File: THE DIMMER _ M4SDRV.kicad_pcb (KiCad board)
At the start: 4 copper layers, 37 x 23.8 mm, 89 parts, among them J1 Conn_01x01, J10 GS2, J2 USB_B_Micro, J3 Conn_01x05, J4 Conn_01x02, J5 Conn_01x01, J6 Conn_01x01, J7 Conn_01x04, J8 Conn_01x02, J9 Conn_01x04, U1 ATSAMD51J19A-M, U10 DRV50153A, U11 DRV50152A, U12 MAX40056_uMAX8, U13 MAX40056_uMAX8, U14 TMC2209-LA, U15 MIC4605-2YMT, U16 MIC4605-2YMT, U2 MIC4605-2YMT, U3 LM2672M-12, U4 BSC0925NDATMA1, U5 BSC0925NDATMA1, U6 BSC0925NDATMA1, U7 MAX40056_uMAX8, U8 NCP170, U9 DRV50152A, Y1 Crystal_GND2_Small

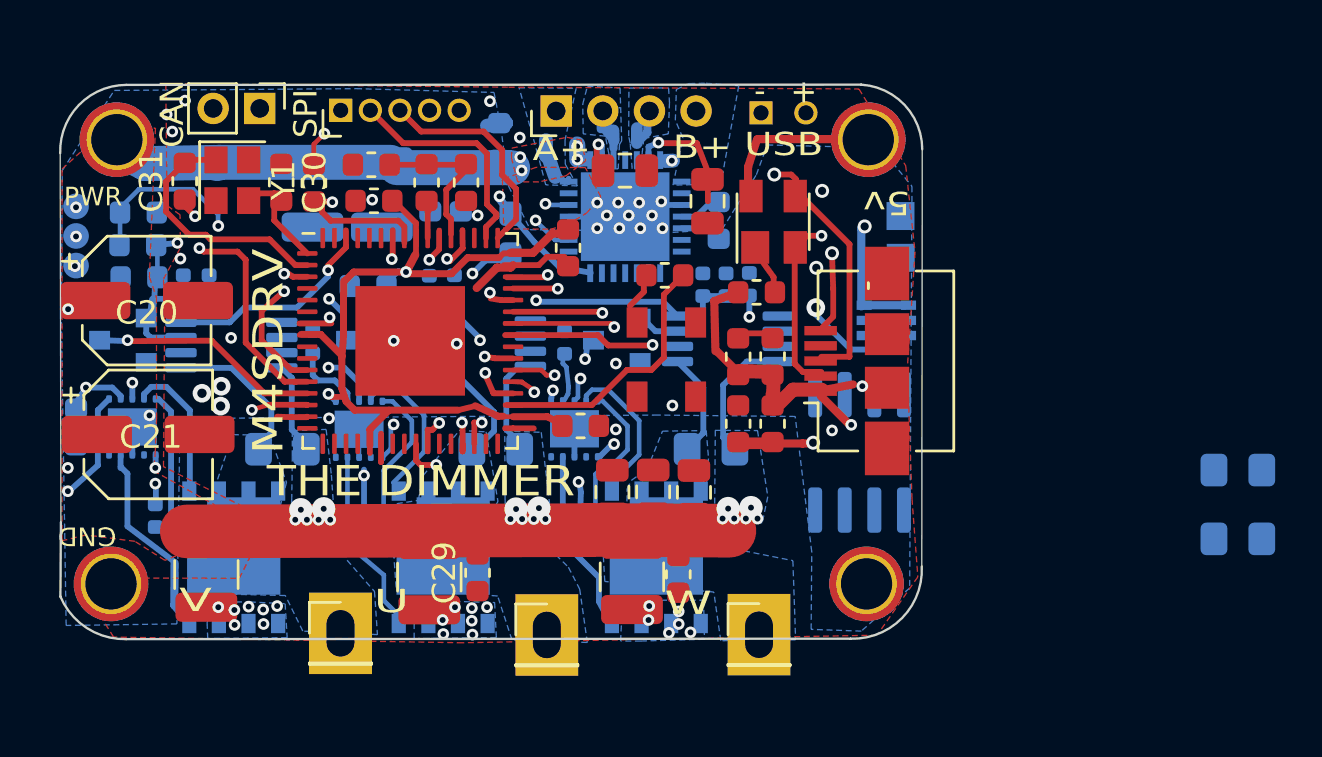
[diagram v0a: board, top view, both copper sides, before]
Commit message: update
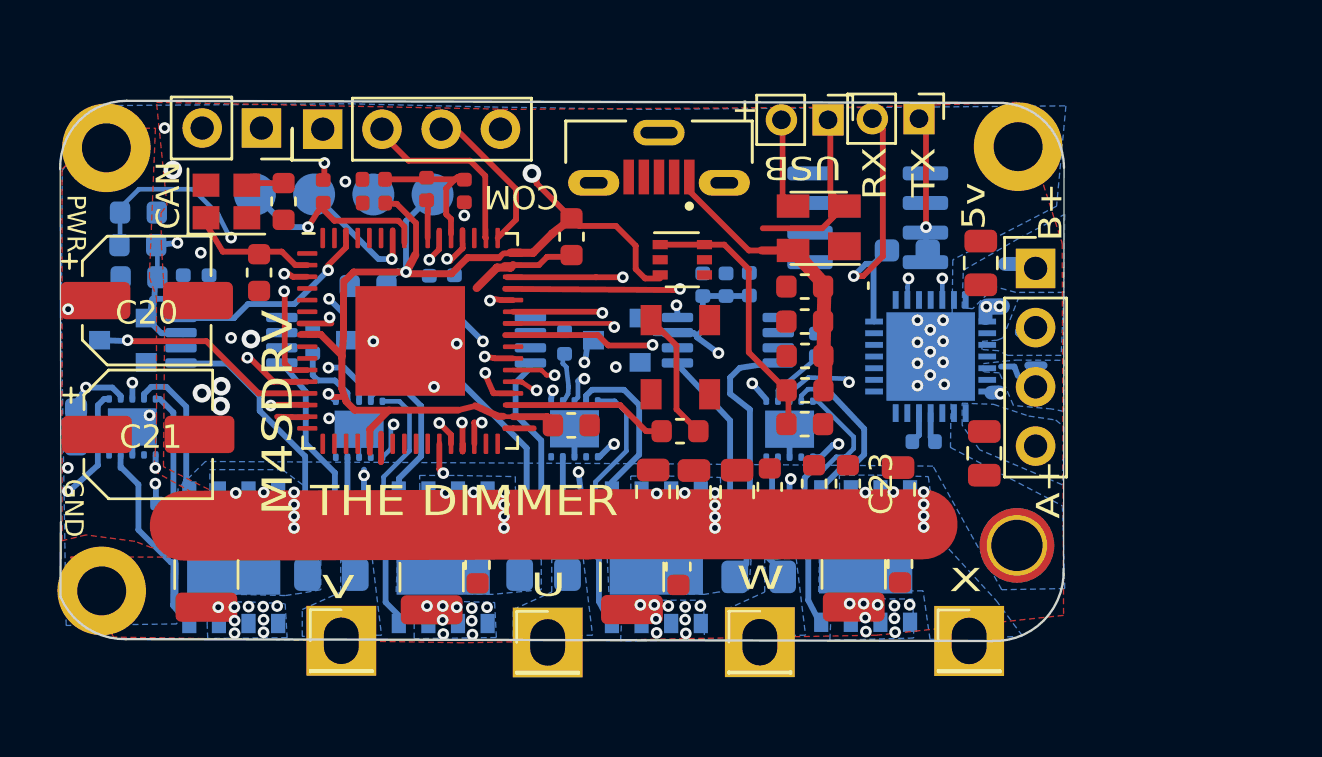
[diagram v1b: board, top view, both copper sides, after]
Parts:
- removed C10, C9: 10uF, Capacitor_SMD:C_1210_3225Metric
- removed C24: 10nF, Capacitor_SMD:C_0603_1608Metric
- removed J10: GS2, LED_SMD:Solder joint
- removed R12, R16: 0.02ohm, Resistor_SMD:R_0805_2012Metric_Pad1.15x1.40mm_HandSolder
- added C22: 1uF7, Capacitor_SMD:C_0603_1608Metric, F.Cu at (94.0, 75.0)
- added C25: 4.7uF, Capacitor_SMD:C_0805_2012Metric, F.Cu at (99.5, 75.1)
- added C28: 1uF, Capacitor_SMD:C_0603_1608Metric, F.Cu at (99.5, 78.3)
- added C44: 1uF, Capacitor_SMD:C_0402_1005Metric, B.Cu at (96.0, 68.9)
- added C45: 1uF, Capacitor_SMD:C_0402_1005Metric, B.Cu at (94.8, 76.5)
- added C8: 10uF, Capacitor_SMD:C_1210_3225Metric, F.Cu at (97.6, 78.7)
- added J11: Conn_01x01, Connector_PinHeader_2.54mm:PinHeader_1x01_P2.54mm_Vertical, F.Cu at (102.5, 81.6)
- added J12: Conn_01x02, Connector_PinHeader_2.00mm:PinHeader_1x02_P2.00mm_Vertical, F.Cu at (100.4, 59.2)
- added U17: MIC4605-2YMT, LED_SMD:MIC4605, B.Cu at (94.8, 72.5)
- added U18: BSC0925NDATMA1, Package_SON:Infineon_PG-TISON-8-2, B.Cu at (99.7, 80.3)
- C11, C16, C19, C2: footprint Capacitor_SMD:C_0603_1608Metric -> Capacitor_SMD:C_0402_1005Metric
- C22, C23, U8: moved to F.Cu
- J2: footprint Connector_USB:USB_Micro-B_Amphenol_10104110_Horizontal -> molex_usb_vert:MOLEX_1051330001
- J3: footprint Connector_PinHeader_1.27mm:PinHeader_1x05_P1.27mm_Vertical -> Connector_PinHeader_2.54mm:PinHeader_1x04_P2.54mm_Vertical
- J4: footprint Connector_PinHeader_2.00mm:PinHeader_1x02_P2.00mm_Vertical -> Connector_PinSocket_2.54mm:PinSocket_1x02_P2.54mm_Vertical
- J7: footprint Connector_PinHeader_2.00mm:PinHeader_1x04_P2.00mm_Vertical -> Connector_PinHeader_2.54mm:PinHeader_1x04_P2.54mm_Vertical
- J8: footprint Connector_PinHeader_1.27mm:PinHeader_1x02_P1.27mm_Vertical -> Connector_PinHeader_2.00mm:PinHeader_1x02_P2.00mm_Vertical
- L1: footprint Inductor_SMD:L_0603_1608Metric -> Inductor_SMD:L_0402_1005Metric
- R6: footprint Resistor_SMD:R_0603_1608Metric -> Resistor_SMD:R_0402_1005Metric
- moved R2 38.9 mm to (75.2, 78.7)
- moved R3 30.1 mm to (84.3, 78.7)
- moved C23 21.8 mm to (97.3, 74.8), turned to -90 degrees
- moved J7 21.6 mm to (105.4, 65.6), turned to 0 degrees
- moved C22 19.9 mm to (95.9, 74.8)
- moved R21 17.0 mm to (99.9, 64.8), turned to 0 degrees
- moved R19 16.1 mm to (103.2, 73.5)
- moved R20 15.8 mm to (103.0, 65.4), turned to -90 degrees
- moved U14 14.4 mm to (100.9, 69.4), turned to 90 degrees
- moved J9 13.1 mm to (77.0, 62.4), turned to 0 degrees
- moved C19 12.9 mm to (100.6, 73.0), turned to 180 degrees
- moved R8 12.5 mm to (93.5, 78.8)
- moved J2 11.4 mm to (89.2, 61.9), turned to 180 degrees
- moved U3 10.1 mm to (98.2, 63.4), turned to 180 degrees
- moved U8 9.13 mm to (90.2, 65.2), turned to 0 degrees
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- renumbered U7 to U12, U12 to U7
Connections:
- net TCC0_CH2/Switch 3 renamed TCC0_CH2/CAN0Switch 3
- R2 pad 1: +12V -> V
- R2 pad 2: +12V -> V
- R3 pad 1: +12V -> U
- R3 pad 2: +12V -> U
- R8 pad 1: +12V -> W
- R8 pad 2: +12V -> W
- U1 pad 25: CAN1_TX -> Net-(U1-Pad25)
- U1 pad 26: CAN1_RX -> CAN1_STANDBY
- U1 pad 27: Net-(U1-Pad27) -> CAN1_TX
- U1 pad 28: Net-(U1-Pad28) -> CAN1_RX
- U12 pad 1: +12V -> V
- U12 pad 8: +12V -> V
- U13 pad 1: +12V -> U
- U13 pad 8: +12V -> U
- U15 pad 11: GND -> (no net)
- U16 pad 11: GND -> (no net)
- U2 pad 11: GND -> (no net)
- U7 pad 1: +12V -> W
- U7 pad 8: +12V -> W
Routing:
- net +12V: track 80.0 -> 44.6 mm, vias 24 -> 29
- net UART_TX: track 11.8 -> 35.4 mm
- net V: track 9.62 -> 31.6 mm
- net W: track 10.8 -> 32.2 mm
- net U: track 11.9 -> 33.3 mm
- net VBUS: track 30.8 -> 12.8 mm, vias 2 -> 0
- net UART_RX: track 17.4 -> 33.0 mm
- net GND: track 31.2 -> 16.8 mm, vias 56 -> 65
- net Net-(C45-Pad1): track 0.00 -> 12.3 mm, vias 0 -> 2
- net X: track 0.00 -> 11.5 mm
- net SWDIO: track 17.1 -> 5.67 mm, vias 2 -> 1
- net SWCLK: track 19.3 -> 8.90 mm, vias 2 -> 1
- net D+: track 28.7 -> 18.8 mm, vias 2 -> 1
- net A3: track 34.2 -> 25.2 mm
- net STEP: track 11.5 -> 20.5 mm
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- added copper zone on B.Cu, net X
- removed copper zone on In1.Cu, net +12V
- removed copper zone on In2.Cu, net +12V
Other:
- board size 37 x 23.8 mm -> 43.1 x 23.2 mm
- board text added: "CLK"
- board text added: "COM"
- board text added: "DIO"
- board text added: "RX"
- board text added: "TX"
- board text added: "X"
- board text removed: "-"
- board text removed: "SPI"

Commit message: Dev.
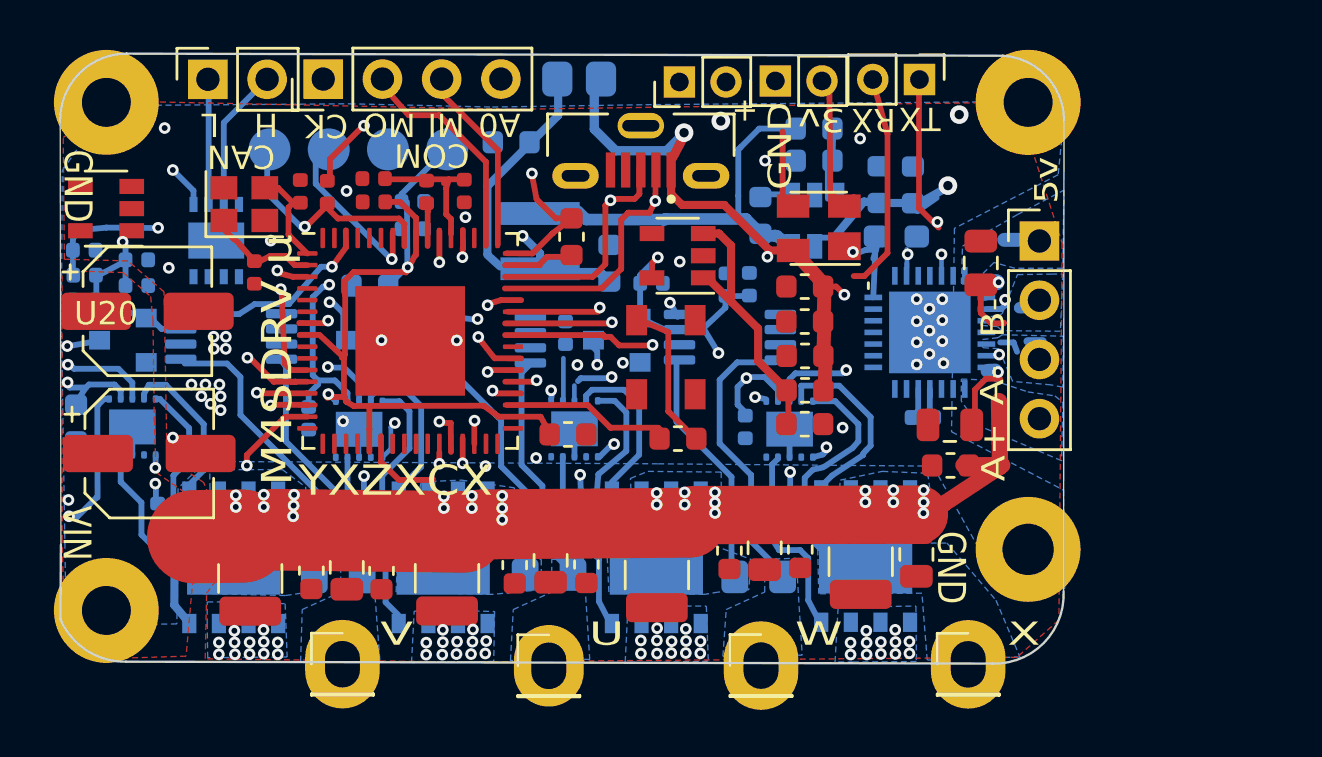
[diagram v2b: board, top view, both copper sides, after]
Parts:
- removed the C8 at (97.6, 78.7)
- added C10: 10uF, Capacitor_SMD:C_1210_3225Metric, F.Cu at (97.9, 78.2)
- added C24: 10nF, Capacitor_SMD:C_0603_1608Metric, F.Cu at (92.2, 77.7)
- added C46: 2.2uF, Capacitor_SMD:C_0603_1608Metric, B.Cu at (98.6, 62.0)
- added C47: 200nF, Capacitor_SMD:C_0603_1608Metric, B.Cu at (100.1, 62.0)
- added C49: 0.1uF, Capacitor_SMD:C_0603_1608Metric, B.Cu at (93.6, 63.3)
- added C50: 200nF, Capacitor_SMD:C_0603_1608Metric, B.Cu at (87.1, 65.4)
- added C51: 200nF, Capacitor_SMD:C_0603_1608Metric, B.Cu at (82.9, 60.2)
- added J10: GS2, Resistor_SMD:R_0805_2012Metric, B.Cu at (85.8, 57.5)
- added J8: Conn_01x02, Connector_PinHeader_2.00mm:PinHeader_1x02_P2.00mm_Vertical, F.Cu at (90.1, 57.6)
- added L2: 33uH, Inductor_SMD:L_Coilcraft_XxL4020, B.Cu at (84.1, 64.4)
- added R1: 100k, Resistor_SMD:R_0603_1608Metric, B.Cu at (95.9, 59.6)
- added R7: 11.11k, Resistor_SMD:R_0603_1608Metric, B.Cu at (95.9, 61.0)
- added U19: MCP2562FD-E_SN, Package_DFN_QFN:DFN-8-1EP_3x3mm_P0.65mm_EP1.55x2.4mm, B.Cu at (70.2, 64.4)
- added U20: LF15_TO220, Package_TO_SOT_SMD:SOT-23-5, F.Cu at (65.5, 63.0)
- C1, C13, C30, C31: footprint Capacitor_SMD:C_0603_1608Metric -> Capacitor_SMD:C_0402_1005Metric
- R5: footprint Resistor_SMD:R_0603_1608Metric -> Resistor_SMD:R_0402_1005Metric
- U10: value DRV50153A -> DRV5053
- U11, U9: value DRV50152A -> DRV5053
- U3: value LM2672M-12 -> LMR50410; footprint Package_SO:SOIC-8_3.9x4.9mm_P1.27mm -> Package_TO_SOT_SMD:SOT-23-6
- U8: value NCP170 -> MIC5219-3.6; footprint Package_TO_SOT_SMD:SOT-363_SC-70-6 -> Package_TO_SOT_SMD:SOT-23-5
- moved C25 23.9 mm to (75.8, 78.4), turned to 90 degrees
- moved H3 21.1 mm to (65.5, 58.4)
- moved C23 20.3 mm to (77.3, 78.6), turned to 90 degrees
- moved C22 20.0 mm to (74.3, 78.6), turned to 90 degrees
- moved H2 19.8 mm to (65.5, 80.3)
- moved C26 8.14 mm to (100.2, 77.9), turned to 90 degrees
- moved C28 7.02 mm to (83.0, 78.3)
- moved C25 6.81 mm to (84.6, 78.1), turned to 90 degrees
- moved C27 5.35 mm to (93.7, 77.6), turned to 90 degrees
- moved C28 4.75 mm to (101.7, 74.1), turned to 0 degrees
- moved C29 4.67 mm to (86.1, 78.3)
- moved C44 4.66 mm to (92.9, 72.4), turned to -90 degrees
- moved C43 4.06 mm to (78.6, 62.7), turned to 180 degrees
- moved C33 3.28 mm to (74.2, 72.0), turned to -90 degrees
- moved J4 3.10 mm to (69.9, 57.5), turned to 90 degrees
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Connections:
- C18 pad 2: +12V -> VIN
- C20 pad 1: +12V -> VIN
- C21 pad 1: +12V -> VIN
- C22 pad 2: +12V -> VIN (x2)
- C23 pad 2: +12V -> VIN
- C25 pad 2: +12V -> VIN (x2)
- C26 pad 2: +12V -> VIN
- C27 pad 2: +12V -> VIN
- C28 pad 2: +12V -> VIN (x2)
- C29 pad 2: +12V -> VIN
- C32 pad 1: +12V -> VOUT/10v
- C33 pad 1: +12V -> VOUT/10v
- C34 pad 1: +12V -> VOUT/10v
- C44 pad 1: +12V -> VOUT/10v
- C7 pad 2: +12V -> VIN
- C8 pad 2: +12V -> VIN
- H2 pad 1: +12V -> VIN
- J4 pad 1: CAN1_RX -> CAN_L
- J4 pad 2: CAN1_TX -> CAN_H
- U14 pad 22: +12V -> VIN
- U14 pad 28: +12V -> VIN
- U15 pad 2: +12V -> VOUT/10v
- U16 pad 2: +12V -> VOUT/10v
- U17 pad 2: +12V -> VOUT/10v
- U18 pad 2: +12V -> VIN
- U2 pad 2: +12V -> VOUT/10v
- U3 pad 1: +12V -> Net-(C49-Pad2)
- U3 pad 2: Net-(U3-Pad2) -> GND
- U3 pad 4: Net-(U3-Pad4) -> VIN
- U3 pad 5: Net-(U3-Pad5) -> VIN
- U3 pad 6: GND -> Net-(C49-Pad1)
- U4 pad 2: +12V -> VIN
- U5 pad 2: +12V -> VIN
- U6 pad 2: +12V -> VIN
- U8 pad 3: +3V3 -> /+5v_filtered
- U8 pad 4: (no net) -> Net-(U8-Pad4)
- U8 pad 5: GND -> +3V3
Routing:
- net VOUT/10v: track 0.00 -> 69.9 mm, vias 0 -> 5
- net VIN: track 0.00 -> 62.3 mm, vias 0 -> 31
- net +12V: track 44.6 -> 0.00 mm, vias 29 -> 0
- net VBUS: track 12.8 -> 35.0 mm, vias 0 -> 3
- net A5: track 2.04 -> 23.9 mm, vias 1 -> 2
- net Net-(C49-Pad1): track 0.00 -> 18.5 mm
- net D+: track 18.8 -> 26.7 mm
- net CAN_H: track 0.00 -> 6.14 mm
- net CAN_L: track 0.00 -> 5.38 mm
- net Net-(C36-Pad1): track 7.03 -> 12.1 mm
- net A3: track 25.2 -> 21.4 mm
- net Net-(R20-Pad2): track 0.00 -> 3.57 mm, vias 0 -> 1
- net +3V3: track 95.2 -> 98.5 mm, vias 10 -> 11
- net Net-(R1-Pad2): track 0.00 -> 3.31 mm
- net Net-(R19-Pad2): track 0.00 -> 3.26 mm, vias 0 -> 1
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- added copper zone on B.Cu, net VIN
- added copper zone on F.Cu, net VIN
- removed copper zone on B.Cu, net +12V
- removed copper zone on F.Cu, net +12V
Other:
- board size 43.1 x 23.2 mm -> 43.1 x 26.2 mm
- board text added: "3V3"
- board text added: "3v"
- board text added: "A-"
- board text added: "A0"
- board text added: "A0/DAC"
- board text added: "B-"
- board text added: "Bridge"
- board text added: "CK"
- board text added: "H"
- board text added: "L"
- board text added: "M4SDRV µ"
- board text added: "MI"
- board text added: "MISO"
- board text added: "MO"
- board text added: "MOSI"
- board text added: "SCK"
- board text added: "VIN"
- board text added: "YXZXCX"
- board text removed: "B+"
- board text removed: "M4SDRV"
- board text removed: "PWR"
- board text removed: "SWO"
- board text removed: "THE DIMMER"
- board text removed: "USB"
